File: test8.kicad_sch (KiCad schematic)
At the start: 4 parts, among them J1 Conn_01x02_Pin, U1 74HC165, U2 74HC165, U3 ESP32-WROOM-32

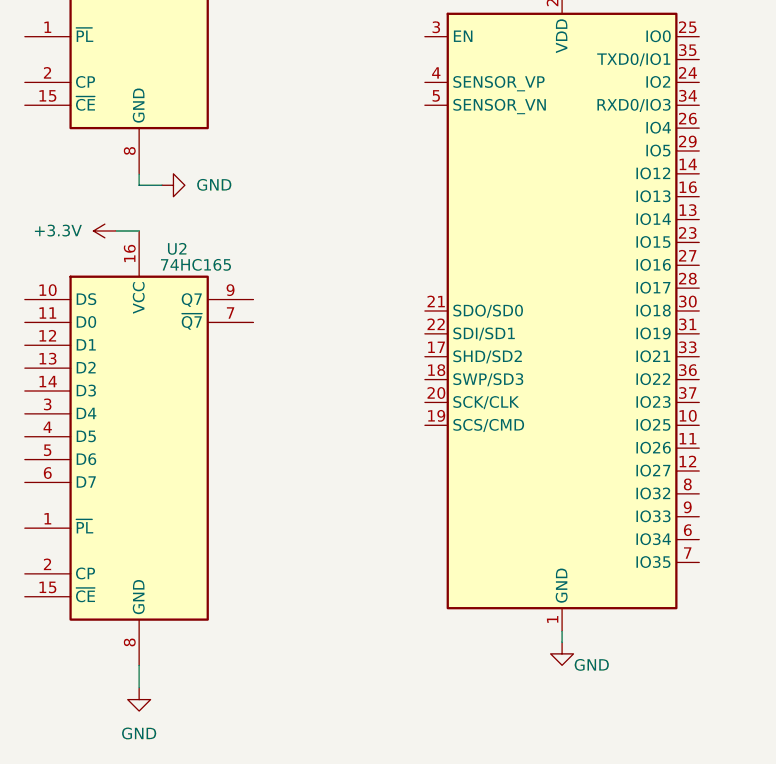
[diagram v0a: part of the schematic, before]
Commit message: process
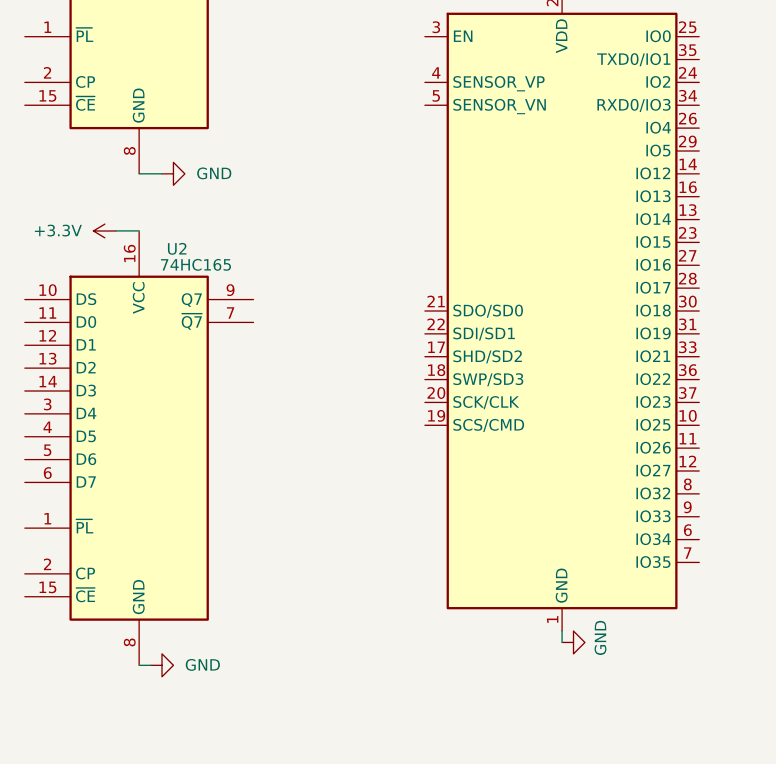
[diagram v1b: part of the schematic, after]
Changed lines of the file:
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@@
 	(wire
 		(pts
-			(xy 78.74 102.87) (xy 78.74 101.6)
+			(xy 125.73 78.74) (xy 125.73 81.28)
 		)
 		(stroke
@@
 	(wire
 		(pts
-			(xy 125.73 78.74) (xy 125.73 81.28)
+			(xy 125.73 152.4) (xy 125.73 153.67)
 		)
 		(stroke
@@
 	(wire
 		(pts
-			(xy 125.73 152.4) (xy 125.73 153.67)
+			(xy 78.74 50.8) (xy 78.74 53.34)
 		)
 		(stroke
@@
 	(wire
 		(pts
-			(xy 78.74 50.8) (xy 78.74 53.34)
+			(xy 111.76 60.96) (xy 111.76 62.23)
 		)
 		(stroke
@@
 	(wire
 		(pts
-			(xy 111.76 60.96) (xy 111.76 62.23)
+			(xy 81.28 101.6) (xy 78.74 101.6)
 		)
 		(stroke
@@
 	(wire
 		(pts
-			(xy 78.74 156.21) (xy 78.74 158.75)
+			(xy 80.01 156.21) (xy 78.74 156.21)
 		)
 		(stroke
@@
 	(wire
 		(pts
-			(xy 81.28 102.87) (xy 78.74 102.87)
+			(xy 114.3 60.96) (xy 114.3 62.23)
 		)
 		(stroke
@@
 		)
 	)
-	(wire
-		(pts
-			(xy 114.3 60.96) (xy 114.3 62.23)
-		)
-		(stroke
-			(width 0)
-			(type default)
-		)
-	)
 	(symbol
 		(lib_id "power:GND")
-		(at 78.74 158.75 0)
+		(at 80.01 156.21 90)
 		(unit 1)
 		(exclude_from_sim no)
@@
 		(fields_autoplaced yes)
 		(property "Reference" "#PWR05"
-			(at 78.74 165.1 0)
+			(at 86.36 156.21 0)
 			(effects
 				(font
@@
 		)
 		(property "Value" "GND"
-			(at 78.74 163.83 0)
-			(effects
-				(font
-					(size 1.27 1.27)
-				)
+			(at 83.82 156.2099 90)
+			(effects
+				(font
+					(size 1.27 1.27)
+				)
+				(justify right)
 			)
 		)
 		(property "Footprint" ""
-			(at 78.74 158.75 0)
+			(at 80.01 156.21 0)
 			(effects
 				(font
@@
 		)
 		(property "Datasheet" ""
-			(at 78.74 158.75 0)
+			(at 80.01 156.21 0)
 			(effects
 				(font
@@
 		)
 		(property "Description" "Power symbol creates a global label with name \"GND\" , ground"
-			(at 78.74 158.75 0)
+			(at 80.01 156.21 0)
 			(effects
 				(font
@@
 	(symbol
 		(lib_id "power:GND")
-		(at 125.73 153.67 0)
+		(at 125.73 153.67 90)
 		(unit 1)
 		(exclude_from_sim no)
@@
 		(dnp no)
 		(property "Reference" "#PWR08"
-			(at 125.73 160.02 0)
+			(at 132.08 153.67 0)
 			(effects
 				(font
@@
 		)
 		(property "Value" "GND"
-			(at 129.032 156.21 0)
+			(at 130.048 153.162 0)
 			(effects
 				(font
@@
 	(symbol
 		(lib_id "power:GND")
-		(at 81.28 102.87 90)
+		(at 81.28 101.6 90)
 		(unit 1)
 		(exclude_from_sim no)
@@
 		(fields_autoplaced yes)
 		(property "Reference" "#PWR02"
-			(at 87.63 102.87 0)
+			(at 87.63 101.6 0)
 			(effects
 				(font
@@
 		)
 		(property "Value" "GND"
-			(at 85.09 102.8699 90)
+			(at 85.09 101.5999 90)
 			(effects
 				(font
@@
 		)
 		(property "Footprint" ""
-			(at 81.28 102.87 0)
+			(at 81.28 101.6 0)
 			(effects
 				(font
@@
 		)
 		(property "Datasheet" ""
-			(at 81.28 102.87 0)
+			(at 81.28 101.6 0)
 			(effects
 				(font
@@
 		)
 		(property "Description" "Power symbol creates a global label with name \"GND\" , ground"
-			(at 81.28 102.87 0)
-			(effects
-				(font
+			(at 81.28 101.6 0)
+			(effects
+				(font

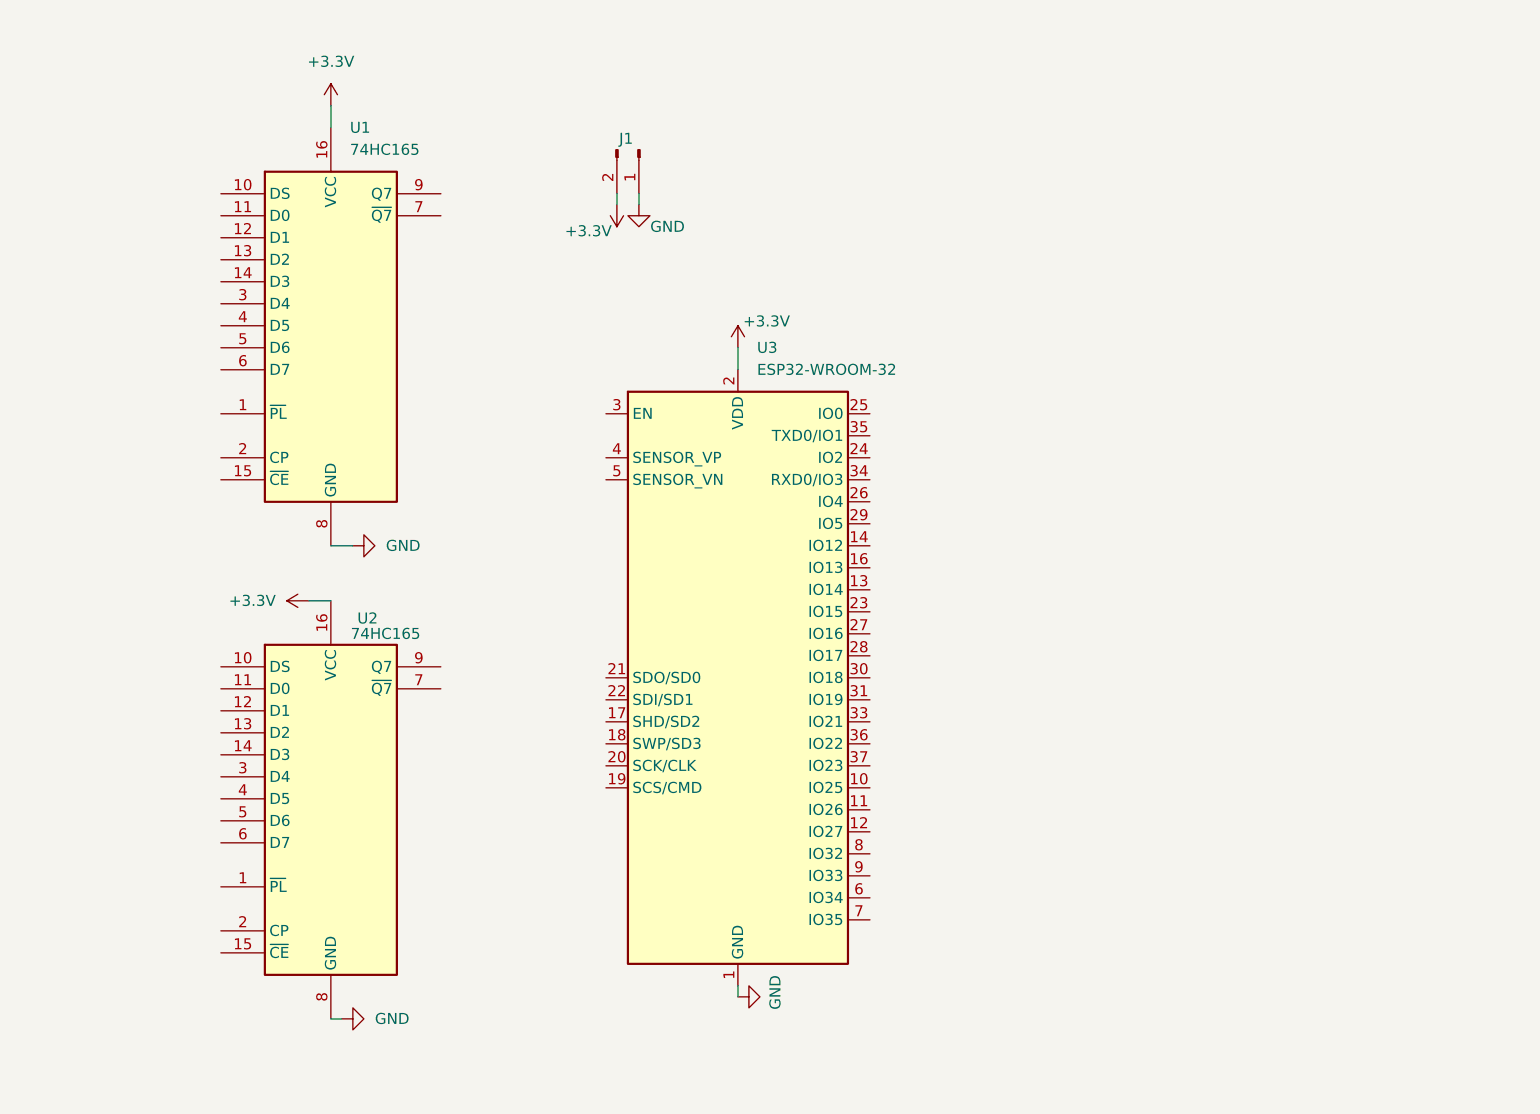
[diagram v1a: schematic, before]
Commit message: xz
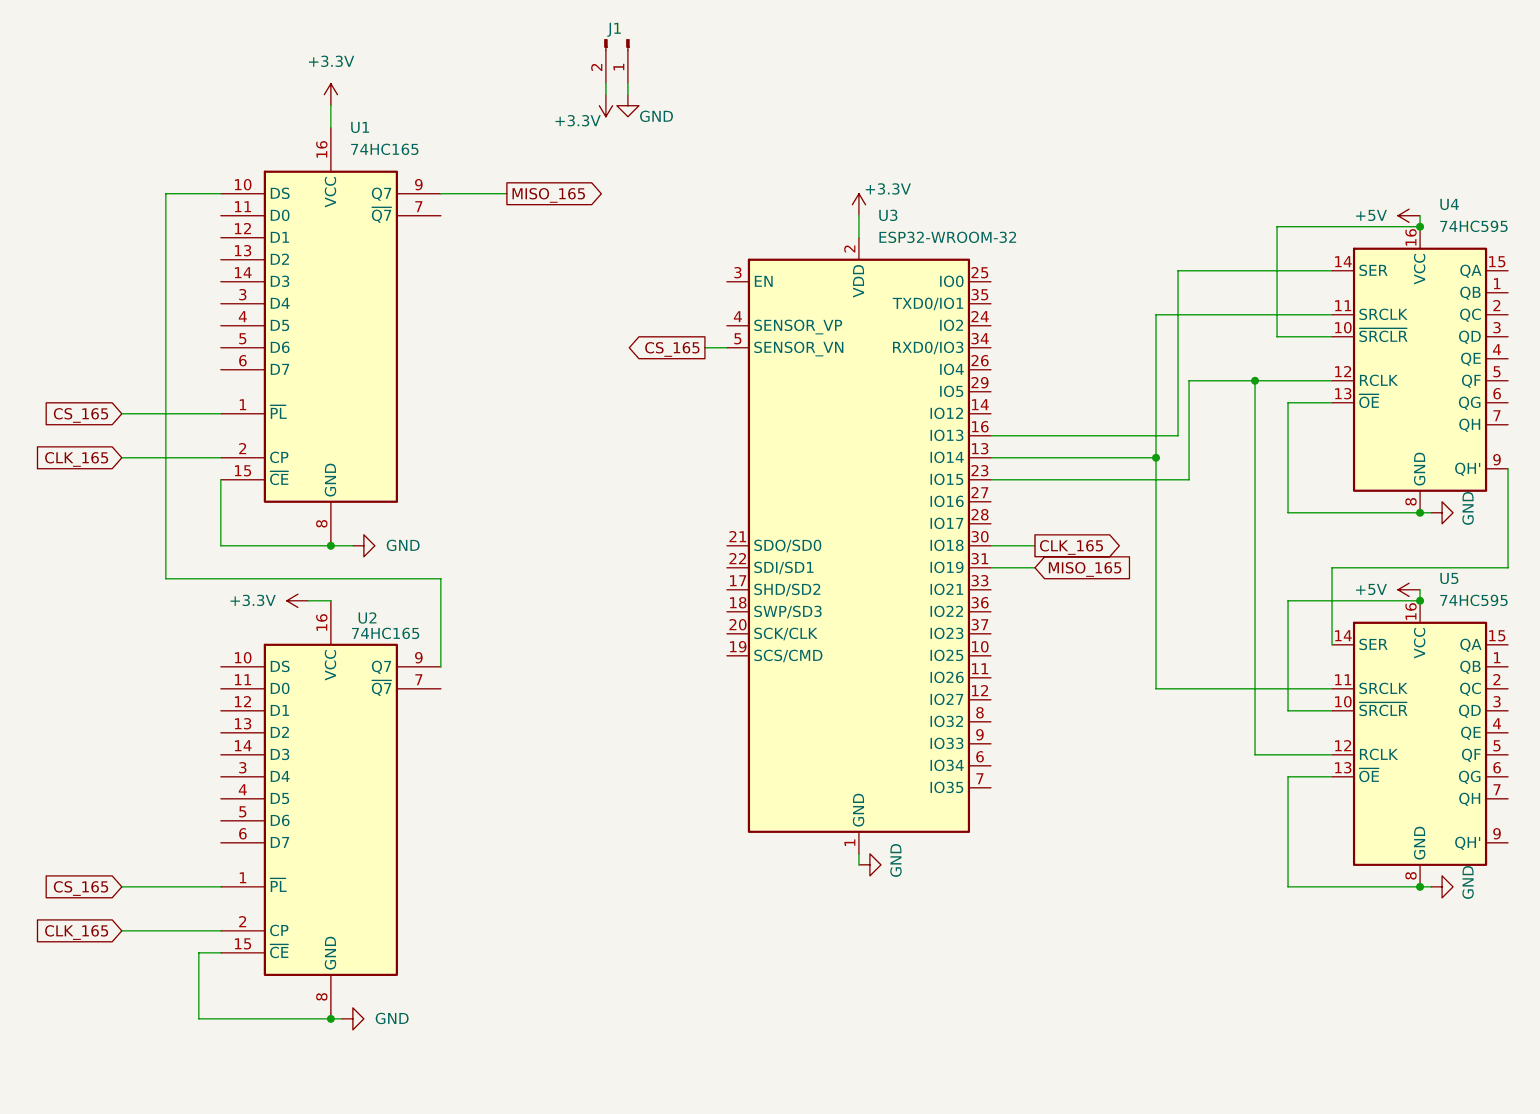
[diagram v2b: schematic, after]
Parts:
- added U4, U5: 74HC595, Package_DIP:DIP-16_W7.62mm_LongPads, symbol 74xx:74HC595
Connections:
- net GND: now also U1.15 (~{CE}), U2.15 (~{CE}), U4.13 (~{OE}), U4.8 (GND), U5.13 (~{OE}), U5.8 (GND)
- net CS_165: now reaches U1.1 (~{PL})
- net CS_165: now also U2.1 (~{PL}), U3.5 (SENSOR_VN)
- net at U1.10 (DS): now also U2.9 (Q7)
- net CLK_165: now reaches U1.2 (CP)
- net CLK_165: now also U2.2 (CP), U3.30 (IO18)
- net MISO_165: now reaches U1.9 (Q7)
- net MISO_165: now also U3.31 (IO19)
- net at U3.13 (IO14): now also U4.11 (SRCLK), U5.11 (SRCLK)
- net at U3.16 (IO13): now also U4.14 (SER)
- net at U3.23 (IO15): now also U4.12 (RCLK), U5.12 (RCLK)
- new net: U4.9 (QH'), U5.14 (SER)
- new net +5V: U4.10 (~{SRCLR}), U4.16 (VCC), U5.10 (~{SRCLR}), U5.16 (VCC)
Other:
- moved on the sheet: J1, U3
